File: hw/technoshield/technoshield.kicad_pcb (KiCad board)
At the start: 2 copper layers, 68.6 x 53.3 mm, 9 parts, among them P1 Power, P2 Analog, P3 Digital, P4 Digital, P5 CONN_1, P6 CONN_1, P7 CONN_1, P8 CONN_1

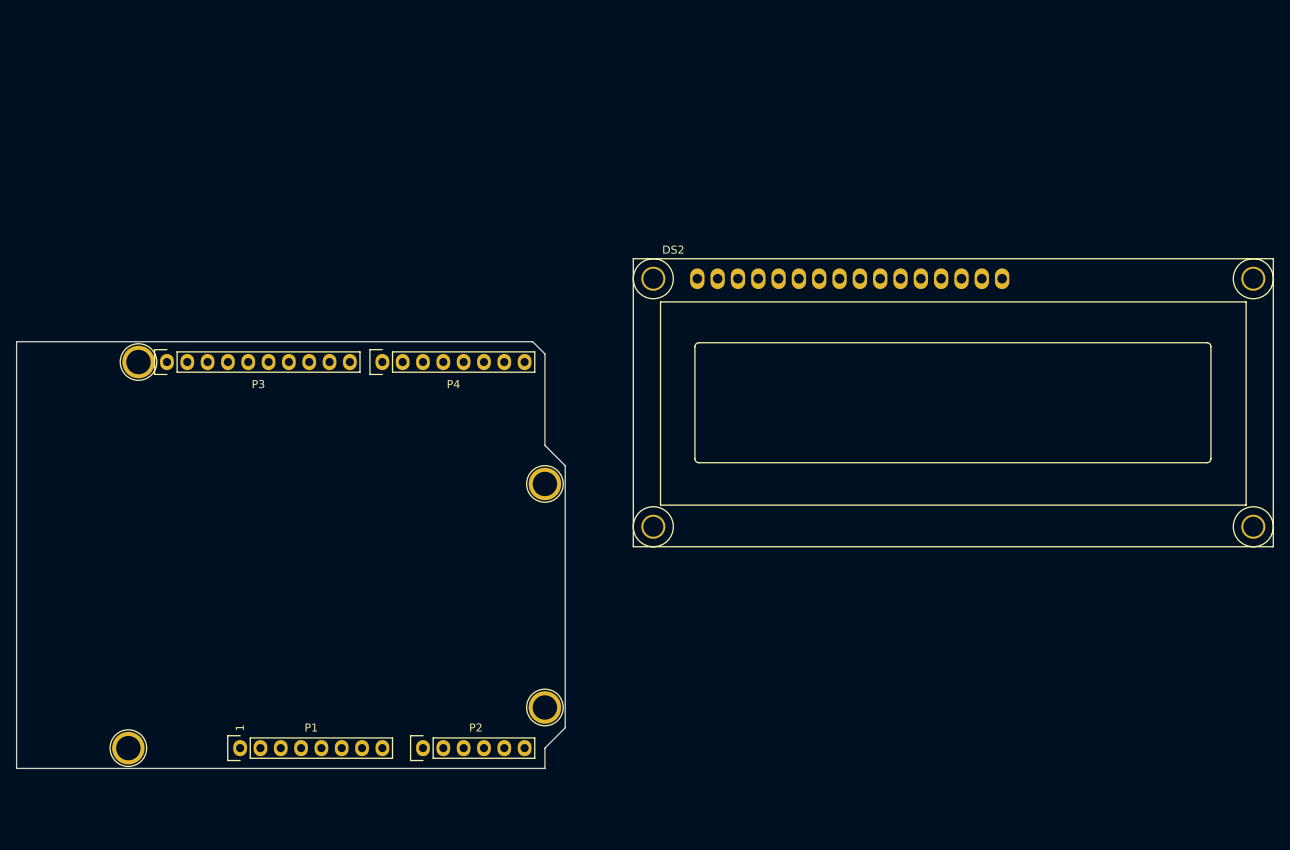
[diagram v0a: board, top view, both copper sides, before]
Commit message: During dev PCB.
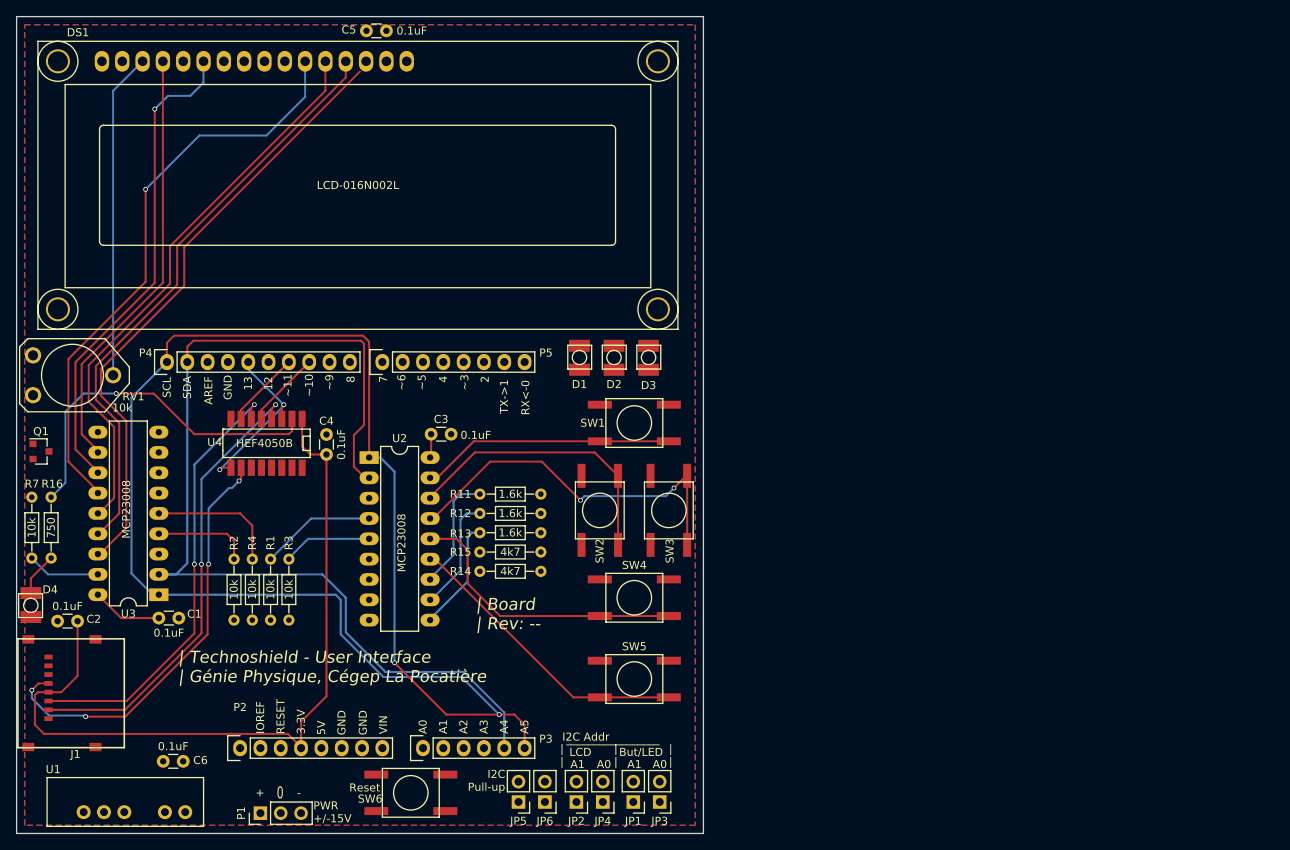
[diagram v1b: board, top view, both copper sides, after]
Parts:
- removed DS2: LCD16X2, Displays:WC1602A
- removed P6, P7, P8: CONN_1, Socket_Arduino_Uno:Arduino_1pin
- added C1: 0.1uF, Capacitors_THT:C_Disc_D3.0mm_W1.6mm_P2.50mm, F.Cu at (128.8, 107.6)
- added C2: 0.1uF, Capacitors_THT:C_Disc_D3.0mm_W1.6mm_P2.50mm, F.Cu at (118.6, 108.0)
- added C3: 0.1uF, Capacitors_THT:C_Disc_D3.0mm_W1.6mm_P2.50mm, F.Cu at (162.8, 84.6)
- added C4: 0.1uF, Capacitors_THT:C_Disc_D3.0mm_W1.6mm_P2.50mm, F.Cu at (149.7, 87.1)
- added C5: 0.1uF, Capacitors_THT:C_Disc_D3.0mm_W1.6mm_P2.50mm, F.Cu at (157.2, 34.2)
- added C6: 0.1uF, Capacitors_THT:C_Disc_D3.0mm_W1.6mm_P2.50mm, F.Cu at (131.8, 125.5)
- added D1: LS T67K-J1K2-1-Z, T67K:T67K, F.Cu at (181.4, 73.5)
- added D2: LY T67K-J2L1-26-Z, T67K:T67K, F.Cu at (185.7, 73.5)
- added D3: LP T67K-E1F2-25-Z, T67K:T67K, F.Cu at (190.0, 73.5)
- added D4: LP T67K-E1F2-25-Z, T67K:T67K, F.Cu at (112.8, 107.4)
- added DS1: LCD-016N002L, Displays:WC1602A, F.Cu at (121.7, 38.0)
- added J1: 101-00303-68-1-ND, Connectors_lib:MICRO_SD_HINGE_AMP, F.Cu at (124.5, 117.0)
- added JP1: JUMPER, Pin_Headers:Pin_Header_Straight_1x02_Pitch2.54mm, F.Cu at (188.1, 130.6)
- added JP2: JUMPER, Pin_Headers:Pin_Header_Straight_1x02_Pitch2.54mm, F.Cu at (181.0, 130.6)
- added JP3: JUMPER, Pin_Headers:Pin_Header_Straight_1x02_Pitch2.54mm, F.Cu at (191.4, 130.6)
- added JP4: JUMPER, Pin_Headers:Pin_Header_Straight_1x02_Pitch2.54mm, F.Cu at (184.3, 130.6)
- added JP5: JUMPER, Pin_Headers:Pin_Header_Straight_1x02_Pitch2.54mm, F.Cu at (173.7, 130.6)
- added JP6: JUMPER, Pin_Headers:Pin_Header_Straight_1x02_Pitch2.54mm, F.Cu at (177.0, 130.6)
- added Q1: MMBT2222A-7-F, TO_SOT_Packages_SMD:SOT-23, F.Cu at (114.0, 86.7)
- added R1: 10k, Resistors_THT:R_Axial_DIN0204_L3.6mm_D1.6mm_P7.62mm_Horizontal, F.Cu at (142.7, 100.2)
- added R11: 1.6k, Resistors_THT:R_Axial_DIN0204_L3.6mm_D1.6mm_P7.62mm_Horizontal, F.Cu at (176.5, 92.1)
- added R12: 1.6k, Resistors_THT:R_Axial_DIN0204_L3.6mm_D1.6mm_P7.62mm_Horizontal, F.Cu at (176.5, 94.5)
- added R13: 1.6k, Resistors_THT:R_Axial_DIN0204_L3.6mm_D1.6mm_P7.62mm_Horizontal, F.Cu at (176.5, 96.9)
- added R14: 4k7, Resistors_THT:R_Axial_DIN0204_L3.6mm_D1.6mm_P7.62mm_Horizontal, F.Cu at (168.9, 101.7)
- added R15: 4k7, Resistors_THT:R_Axial_DIN0204_L3.6mm_D1.6mm_P7.62mm_Horizontal, F.Cu at (168.9, 99.3)
- added R16: 750, Resistors_THT:R_Axial_DIN0204_L3.6mm_D1.6mm_P7.62mm_Horizontal, F.Cu at (115.3, 100.1)
- added R2: 10k, Resistors_THT:R_Axial_DIN0204_L3.6mm_D1.6mm_P7.62mm_Horizontal, F.Cu at (138.2, 100.2)
- added R3: 10k, Resistors_THT:R_Axial_DIN0204_L3.6mm_D1.6mm_P7.62mm_Horizontal, F.Cu at (145.0, 100.2)
- added R4: 10k, Resistors_THT:R_Axial_DIN0204_L3.6mm_D1.6mm_P7.62mm_Horizontal, F.Cu at (140.5, 100.2)
- added R7: 10k, Resistors_THT:R_Axial_DIN0204_L3.6mm_D1.6mm_P7.62mm_Horizontal, F.Cu at (112.9, 92.5)
- added REF***: OSHW-Symbol_13.4x12mm_SilkScreen, Symbols:OSHW-Symbol_13.4x12mm_SilkScreen, B.Cu at (152.1, 54.2)
- added RV1: 10k, POTENTIOMETRES:POTENTIOMETRE_BOURNS_3319P, F.Cu at (123.1, 77.2)
- added SW1: SW_PUSH, smt_btn:smt_btn, F.Cu at (183.6, 85.2)
- added SW2: SW_PUSH, smt_btn:smt_btn, F.Cu at (185.9, 98.7)
- added SW3: SW_PUSH, smt_btn:smt_btn, F.Cu at (194.6, 98.7)
- added SW4: SW_PUSH, smt_btn:smt_btn, F.Cu at (183.6, 107.1)
- added SW5: SW_PUSH, smt_btn:smt_btn, F.Cu at (183.6, 117.2)
- added SW6: SW_PUSH, smt_btn:smt_btn, F.Cu at (155.7, 131.4)
- added U1: PDM1-S5-D15-S, PDM1-S:PDM1-S, F.Cu at (124.5, 131.8)
- added U2: MCP23008, Housings_DIP:DIP-18_W7.62mm_LongPads, F.Cu at (155.1, 87.5)
- added U3: MCP23008, Housings_DIP:DIP-18_W7.62mm_LongPads, F.Cu at (128.8, 104.6)
- added U4: HEF4050B, SO16-3_9mm:SO16-3_9mm, F.Cu at (138.4, 93.9)
- P1: value Power -> CONN_01X03; footprint Socket_Arduino_Uno:Socket_Strip_Arduino_1x08 -> Pin_Headers:Pin_Header_Straight_1x03_Pitch2.54mm
- P2: value Analog -> Power; footprint Socket_Arduino_Uno:Socket_Strip_Arduino_1x06 -> Socket_Arduino_Uno:Socket_Strip_Arduino_1x08
- P3: value Digital -> Analog; footprint Socket_Arduino_Uno:Socket_Strip_Arduino_1x10 -> Socket_Arduino_Uno:Socket_Strip_Arduino_1x06
- P4: footprint Socket_Arduino_Uno:Socket_Strip_Arduino_1x08 -> Socket_Arduino_Uno:Socket_Strip_Arduino_1x10
- P5: value CONN_1 -> Digital; footprint Socket_Arduino_Uno:Arduino_1pin -> Socket_Arduino_Uno:Socket_Strip_Arduino_1x08
- moved P3 57.9 mm to (161.8, 123.8)
- moved P5 57.8 mm to (156.7, 75.6)
- moved P4 26.9 mm to (129.8, 75.6)
- moved P2 22.9 mm to (138.9, 123.8)
- moved P1 8.52 mm to (141.5, 132.0), turned to 90 degrees
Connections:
- P1 pad 2: /IOREF -> Net-(P1-Pad2)
- P1 pad 3: /Reset -> Net-(P1-Pad3)
- P2 pad 1: /A0 -> Net-(P2-Pad1)
- P2 pad 2: /A1 -> /IOREF
- P2 pad 3: /A2 -> /Reset
- P2 pad 4: /A3 -> +3V3
- P2 pad 5: /A4(SDA) -> +5V
- P2 pad 6: /A5(SCL) -> GND
- P3 pad 1: /A5(SCL) -> /A0
- P3 pad 2: /A4(SDA) -> /A1
- P3 pad 3: /AREF -> /A2
- P3 pad 4: GND -> /A3
- P3 pad 5: /13(SCK) -> /A4(SDA)
- P3 pad 6: /12(MISO) -> /A5(SCL)
- P4 pad 1: /7 -> /A5(SCL)
- P4 pad 2: /6(**) -> /A4(SDA)
- P4 pad 3: /5(**) -> /AREF
- P4 pad 4: /4 -> GND
- P4 pad 5: /3(**) -> /13(SCK)
- P4 pad 6: /2 -> /12(MISO)
- P4 pad 7: /1(Tx) -> /11(**/MOSI)
- P4 pad 8: /0(Rx) -> /10(**/SS)
- P5 pad 1: Net-(P5-Pad1) -> /7
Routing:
- net /A5(SCL): track 0.00 -> 177.1 mm, vias 0 -> 2
- net /A4(SDA): track 0.00 -> 130.1 mm
- net +3V3: track 0.00 -> 96.3 mm
- net Net-(DS1-Pad14): track 0.00 -> 76.7 mm
- net Net-(DS1-Pad13): track 0.00 -> 74.4 mm
- net Net-(DS1-Pad11): track 0.00 -> 72.7 mm, vias 0 -> 1
- net Net-(DS1-Pad12): track 0.00 -> 71.0 mm
- net Net-(DS1-Pad6): track 0.00 -> 60.9 mm, vias 0 -> 1
- net Net-(D4-Pad1): track 0.00 -> 57.5 mm, vias 0 -> 2
- net Net-(J1-Pad3): track 0.00 -> 55.4 mm, vias 0 -> 2
- net Net-(DS1-Pad4): track 0.00 -> 53.9 mm
- net Net-(J1-Pad5): track 0.00 -> 53.4 mm, vias 0 -> 4
- net Net-(SW3-Pad1): track 0.00 -> 47.0 mm, vias 0 -> 2
- net Net-(R16-Pad2): track 0.00 -> 44.5 mm, vias 0 -> 1
- net Net-(DS1-Pad3): track 0.00 -> 40.8 mm
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- added copper zone on F.Cu, net +5V
- added copper zone on B.Cu, net GND
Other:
- board size 68.6 x 53.3 mm -> 85.9 x 102.1 mm
- board text added: "+"
- board text added: "-"
- board text added: "0"
- board text added: "12"
- board text added: "13"
- board text added: "2"
- board text added: "3.3V"
- board text added: "4"
- board text added: "5V"
- board text added: "7"
- board text added: "8"
- board text added: "A0"
- board text added: "A1"
- board text added: "A2"
- board text added: "A3"
- board text added: "A4"
- board text added: "A5"
- board text added: "AREF"
- board text added: "But/LED"
- board text added: "GND"
- board text added: "I2C Addr"
- board text added: "I2C Pull-up"
- board text added: "IOREF"
- board text added: "LCD"
- board text added: "PWR +/-15V"
- board text added: "RESET"
- board text added: "RX<-0"
- board text added: "Reset"
- board text added: "SCL"
- board text added: "SDA"
- board text added: "TX->1"
- board text added: "Technoshield - User Interface Dépertement de Génie Physique Cégep La Poactière"
- board text added: "VIN"
- board text added: "_________________"
- board text added: "| Board | Rev: --"
- board text added: "| Technoshield - User Interface | Génie Physique, Cégep La Pocatière"
- board text added: "| |"
- board text added: "~~10"
- board text added: "~~11"
- board text added: "~~3"
- board text added: "~~5"
- board text added: "~~6"
- board text added: "~~9"
- board text removed: "1"
